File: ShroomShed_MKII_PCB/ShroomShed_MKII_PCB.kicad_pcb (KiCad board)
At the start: 4 copper layers, 70 x 70 mm, 69 parts, among them J1 SWD 14 pin header, J2 TYPE-C-31-M-12, J3 Fan, J4 AUX_SPI, J5 SD_SPI, J6 DHT_I2C, J7 Display_Touch_SPI, J8 Transducer Driver, J9 Control_Panel, Q1 T2N7002AK, Q2 BC817, SW1 EVQ-Q2B03W, SW2 SW_SPDT, U1 AMS1117-3.3, U2 TPS61085DGK, U3 USBLC6-2SC6, U4 ENS210, U5 STM32H562VGTx, Y1 16MHz

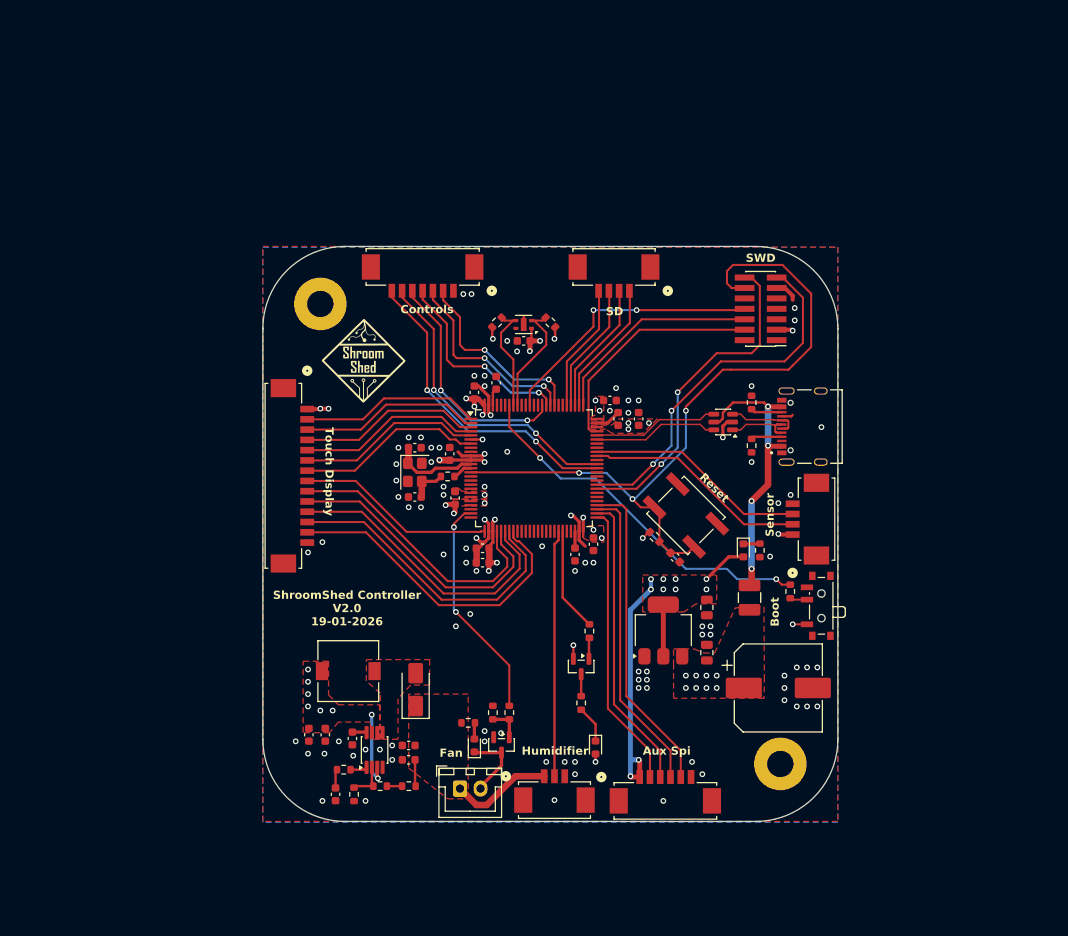
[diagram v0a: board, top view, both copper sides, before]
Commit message: finished V2.1 PCB
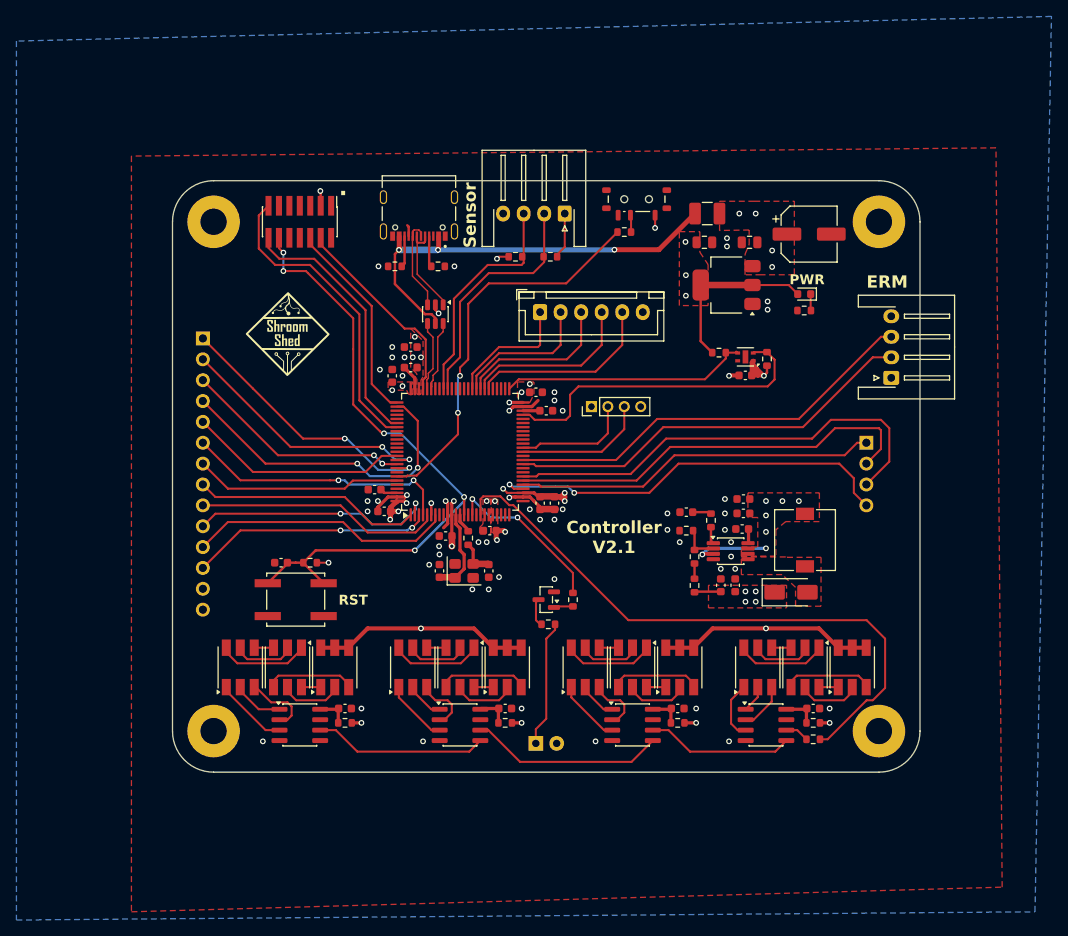
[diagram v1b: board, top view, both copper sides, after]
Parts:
- removed the J4 at (164.0, 132.5)
- removed the J8 at (150.5, 132.4)
- removed J9: Control_Panel, DOWNLOAD_Connectors:CONN_532610001-SD_07_MOL
- removed Q2: BC817, Package_TO_SOT_SMD:SOT-23
- removed the R7 at (150.0, 74.2)
- added C2: 1uF, Capacitor_SMD:C_0603_1608Metric, F.Cu at (182.0, 121.3)
- added C3: 1uF, Capacitor_SMD:C_0603_1608Metric, F.Cu at (125.0, 121.3)
- added C7: 1uF, Capacitor_SMD:C_0603_1608Metric, F.Cu at (165.5, 121.3)
- added C8: 1uF, Capacitor_SMD:C_0603_1608Metric, F.Cu at (144.5, 121.3)
- added D1: XL-5050RGBC, LED_SMD:LED_RGB_5050-6, F.Cu at (186.8, 116.2)
- added D10: XL-5050RGBC, LED_SMD:LED_RGB_5050-6, F.Cu at (154.3, 116.3)
- added D11: XL-5050RGBC, LED_SMD:LED_RGB_5050-6, F.Cu at (144.7, 116.3)
- added D12: XL-5050RGBC, LED_SMD:LED_RGB_5050-6, F.Cu at (139.0, 116.3)
- added D13: XL-5050RGBC, LED_SMD:LED_RGB_5050-6, F.Cu at (133.2, 116.3)
- added D14: BLUE, LED_THT:LED_D4.0mm, B.Cu at (148.2, 125.5)
- added D2: XL-5050RGBC, LED_SMD:LED_RGB_5050-6, F.Cu at (181.0, 116.2)
- added D5: XL-5050RGBC, LED_SMD:LED_RGB_5050-6, F.Cu at (118.0, 116.2)
- added D6: XL-5050RGBC, LED_SMD:LED_RGB_5050-6, F.Cu at (112.2, 116.2)
- added D8: XL-5050RGBC, LED_SMD:LED_RGB_5050-6, F.Cu at (165.8, 116.3)
- added D9: XL-5050RGBC, LED_SMD:LED_RGB_5050-6, F.Cu at (160.0, 116.3)
- added H1: MountingHole_Pad, MountingHole:MountingHole_3.2mm_M3_Pad, F.Cu at (190.0, 62.0)
- added H4: MountingHole_Pad, MountingHole:MountingHole_3.2mm_M3_Pad, F.Cu at (109.0, 124.0)
- added J2: UART, Connector_PinHeader_2.00mm:PinHeader_1x04_P2.00mm_Vertical, F.Cu at (155.0, 84.5)
- added J6: ERM, Connector_JST:JST_XH_S4B-XH-A-1_1x04_P2.50mm_Horizontal, F.Cu at (191.5, 81.0)
- added R1: 33r, Resistor_SMD:R_0603_1608Metric, F.Cu at (182.0, 125.0)
- added R11: 4k7, Resistor_SMD:R_0603_1608Metric, F.Cu at (144.5, 123.0)
- added R20: 10k, Resistor_SMD:R_0603_1608Metric, F.Cu at (145.8, 66.2)
- added R3: 4k7, Resistor_SMD:R_0603_1608Metric, F.Cu at (182.0, 123.0)
- added R4: 4k7, Resistor_SMD:R_0603_1608Metric, F.Cu at (125.0, 123.0)
- added U1: WS2811, Package_SO:SOIC-8_3.9x4.9mm_P1.27mm, F.Cu at (176.2, 123.2)
- added U2: WS2811, Package_SO:SOIC-8_3.9x4.9mm_P1.27mm, F.Cu at (119.5, 123.2)
- added U5: WS2811, Package_SO:SOIC-8_3.9x4.9mm_P1.27mm, F.Cu at (160.0, 123.2)
- added U6: WS2811, Package_SO:SOIC-8_3.9x4.9mm_P1.27mm, F.Cu at (139.0, 123.2)
- C15: renamed from C11; value 1000uF -> 470uF; footprint Capacitor_SMD:CP_Elec_10x10.5 -> Capacitor_SMD:CP_Elec_6.3x7.7
- D3: value Blue -> XL-5050RGBC; footprint LED_SMD:LED_0603_1608Metric -> LED_SMD:LED_RGB_5050-6
- D4: value Yellow -> XL-5050RGBC; footprint LED_SMD:LED_0603_1608Metric -> LED_SMD:LED_RGB_5050-6
- J3: value Fan -> Inputs; footprint Connector_JST:JST_XH_B2B-XH-A_1x02_P2.50mm_Vertical -> Connector_JST:JST_XH_B6B-XH-A_1x06_P2.50mm_Vertical
- J4: renamed from J6; value DHT_I2C -> SHT31; footprint DOWNLOAD_Connectors:CONN_532610001-SD_04_MOL -> Connector_JST:JST_XH_S4B-XH-A-1_1x04_P2.50mm_Horizontal
- J7: renamed from J5; footprint DOWNLOAD_Connectors:CONN_532610001-SD_04_MOL -> Connector_PinSocket_2.54mm:PinSocket_1x04_P2.54mm_Vertical; moved to B.Cu
- J8: renamed from J7; footprint DOWNLOAD_Connectors:CONN_532610001-SD_14_MOL -> Connector_PinSocket_2.54mm:PinSocket_1x14_P2.54mm_Vertical; moved to B.Cu
- Q1: value T2N7002AK -> BC817
- R10: value 2k2 -> 4k7
- R12: value 1k -> 5k1
- R13: value 330r -> 5k1
- R15: value 100R -> 1k
- R16: value 10k -> 500r
- R17: value 2k2 -> 10k
- R18: renamed from R9; value 47r -> 33r
- SW2: value SW_SPDT -> BOOT SELECT; footprint Button_Switch_SMD:SW_SPDT_PCM12 -> Button_Switch_SMD:SW_SPDT_Shouhan_MSK12C02
- moved H2 95.5 mm to (109.0, 62.0)
- moved H3 85.6 mm to (190.0, 124.0)
- moved C1 60.2 mm to (173.5, 95.8), turned to 0 degrees
- moved J3 58.8 mm to (148.8, 73.0)
- moved L1 57.8 mm to (181.0, 100.8), turned to -90 degrees
- moved C4 57.6 mm to (173.5, 97.5), turned to 0 degrees
- moved J5 57.1 mm to (119.5, 62.0), turned to -90 degrees
- moved J1 56.3 mm to (134.0, 59.0), turned to 180 degrees
- moved C15 55.4 mm to (181.5, 63.5)
- moved C6 54.8 mm to (166.6, 97.3), turned to 0 degrees
- moved R12 54.4 mm to (170.5, 77.9), turned to 180 degrees
- moved SW2 54.2 mm to (160.5, 59.2), turned to 180 degrees
- moved R5 54.0 mm to (169.6, 98.3), turned to 90 degrees
- moved C5 53.9 mm to (173.3, 99.4), turned to 0 degrees
- moved R10 53.5 mm to (165.5, 123.0), turned to 180 degrees
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- renumbered C12 to C1, C15 to C10, C10 to C11, C20 to C12, C21 to C13, C22 to C14, C8 to C16, C9 to C17, C23 to C18, C24 to C19, C7 to C20, C1 to C21, C16 to C22, C2 to C23, C3 to C24, C17 to C25, C4 to C26, C5 to C27, C6 to C28, C13 to C4, C18 to C5, C19 to C6, C14 to C9, D1 to D15, D2 to D7, H1 to H3, J2 to J1, J1 to J5, R3 to R14, R14 to R19, R8 to R2, R4 to R21, R11 to R6, R1 to R7, R6 to R8, R2 to R9, U2 to U3, U3 to U4, U4 to U7, U1 to U8, U5 to U9
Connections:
- D3 pad 1: Net-(D3-K) -> Net-(D3-RK)
- D3 pad 2: +5V -> Net-(D3-GK)
- D4 pad 1: Net-(D4-K) -> Net-(D4-RK)
- D4 pad 2: Net-(D4-A) -> Net-(D4-GK)
- J3 pad 1: +12V -> ENCODER_CHANNEL_A
- J3 pad 2: Net-(D4-K) -> ENCODER_CHANNEL_B
- J7 pad 1: SD_NSS -> SD_SCK
- J7 pad 2: SD_SCK -> SD_MISO
- J7 pad 3: SD_MISO -> SD_MOSI
- J7 pad 4: SD_MOSI -> SD_NSS
- J8 pad 1: +3V3 -> TOUCH_IRQ
- J8 pad 10: TOUCH_SCK -> DISPLAY_DC
- J8 pad 11: TOUCH_MISO -> DISPLAY_RST
- J8 pad 12: TOUCH_MOSI -> DISPLAY_NSS
- J8 pad 13: TOUCH_IRQ -> GND
- J8 pad 14: GND -> +3V3
- J8 pad 2: DISPLAY_SCK -> TOUCH_MISO
- J8 pad 3: DISPLAY_DC -> TOUCH_MOSI
- J8 pad 4: DISPLAY_NSS -> TOUCH_NSS
- J8 pad 5: DISPLAY_MISO -> TOUCH_SCK
- J8 pad 6: DISPLAY_MOSI -> DISPLAY_MISO
- J8 pad 7: DISPLAY_RST -> DISPLAY_LED
- J8 pad 8: DISPLAY_LED -> DISPLAY_SCK
- J8 pad 9: TOUCH_NSS -> DISPLAY_MOSI
- Q1 pad 1: Net-(Q1-G) -> Net-(Q1-B)
- Q1 pad 3: Net-(D4-K) -> Net-(Q1-C)
- R10 pad 1: ENS210_SDA -> +12V
- R10 pad 2: +3V3 -> Net-(U5-VDD)
- R12 pad 1: +12V -> ENS210_SDA
- R12 pad 2: Net-(D4-A) -> +3V3
- R13 pad 1: Net-(Q2-C) -> ENS210_SCL
- R13 pad 2: Net-(D3-K) -> +3V3
- R15 pad 1: Net-(Q1-G) -> Net-(Q1-B)
- R15 pad 2: FAN_PWM -> WATER_LED
- R16 pad 1: GND -> Net-(D14-K)
- R16 pad 2: Net-(Q1-G) -> Net-(Q1-C)
- R17 pad 1: Net-(Q2-B) -> +3V3
- R17 pad 2: LED_HUMIDIFIER -> SHT31_SDA
- U9 pad 16: unconnected-(U5-PC1-Pad16) -> WATER_LED
- U9 pad 18: unconnected-(U5-PC3-Pad18) -> RGB_MOSI
- U9 pad 24: FAN_PWM -> unconnected-(U9-PA1-Pad24)
- U9 pad 25: FAN_DETECT -> unconnected-(U9-PA2-Pad25)
- U9 pad 26: DISPLAY_LED -> unconnected-(U9-PA3-Pad26)
- U9 pad 29: TOUCH_NSS -> SD_NSS
- U9 pad 30: TOUCH_SCK -> SD_SCK
- U9 pad 31: TOUCH_MISO -> SD_MISO
- U9 pad 32: TOUCH_MOSI -> SD_MOSI
- U9 pad 33: TOUCH_IRQ -> unconnected-(U9-PC4-Pad33)
- U9 pad 35: unconnected-(U5-PB0-Pad35) -> TRANSDUCER_PWM
- U9 pad 36: unconnected-(U5-PB1-Pad36) -> FAN_PWM
- U9 pad 38: unconnected-(U5-PE7-Pad38) -> RF_RX
- U9 pad 39: unconnected-(U5-PE8-Pad39) -> RF_TX
- U9 pad 44: TRANSDUCER_PWM -> unconnected-(U9-PE13-Pad44)
- U9 pad 45: LED_HUMIDIFIER -> unconnected-(U9-PE14-Pad45)
- U9 pad 47: unconnected-(U5-PB10-Pad47) -> ENS210_SCL
- U9 pad 51: SPI2_NSS -> ENS210_SDA
- U9 pad 52: SPI2_SCK -> unconnected-(U9-PB13-Pad52)
- U9 pad 53: SPI2_MISO -> unconnected-(U9-PB14-Pad53)
- U9 pad 54: SPI2_MOSI -> unconnected-(U9-PB15-Pad54)
- U9 pad 56: unconnected-(U5-PD9-Pad56) -> INPUT_3
- U9 pad 57: unconnected-(U5-PD10-Pad57) -> INPUT_2
- U9 pad 58: UART4_RX -> INPUT_1
- U9 pad 59: UART4_TX -> ENCODER_CHANNEL_B
- U9 pad 60: unconnected-(U5-PD13-Pad60) -> ENCODER_CHANNEL_A
- U9 pad 63: ENCODER_CHANNEL_B -> unconnected-(U9-PC6-Pad63)
- U9 pad 64: ENCODER_CHANNEL_A -> unconnected-(U9-PC7-Pad64)
- U9 pad 77: SD_NSS -> TOUCH_NSS
- U9 pad 78: SD_SCK -> unconnected-(U9-PC10-Pad78)
- U9 pad 79: SD_MISO -> unconnected-(U9-PC11-Pad79)
- U9 pad 80: SD_MOSI -> unconnected-(U9-PC12-Pad80)
- U9 pad 81: unconnected-(U5-PD0-Pad81) -> UART4_RX
- U9 pad 82: unconnected-(U5-PD1-Pad82) -> UART4_TX
- U9 pad 83: LED_WATER -> unconnected-(U9-PD2-Pad83)
- U9 pad 84: BUTTON_2 -> unconnected-(U9-PD3-Pad84)
- U9 pad 85: BUTTON_1 -> unconnected-(U9-PD4-Pad85)
- U9 pad 86: ENCODER_BUTTON -> unconnected-(U9-PD5-Pad86)
- U9 pad 89: SWD_SWO -> TOUCH_SCK
- U9 pad 90: unconnected-(U5-PB4(NJTRST)-Pad90) -> TOUCH_MISO
- U9 pad 91: unconnected-(U5-PB5-Pad91) -> TOUCH_MOSI
- U9 pad 92: ENS210_SCL -> TOUCH_IRQ
- U9 pad 93: ENS210_SDA -> unconnected-(U9-PB7-Pad93)
- U9 pad 95: unconnected-(U5-PB8-Pad95) -> DISPLAY_LED
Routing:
- net RGB_MOSI: track 0.00 -> 75.0 mm
- net +12V: track 15.8 -> 61.5 mm, vias 0 -> 10
- net SD_MOSI: track 15.4 -> 55.9 mm
- net SPI2_MOSI: track 39.1 -> 0.00 mm
- net SPI2_MISO: track 37.7 -> 0.00 mm
- net SPI2_SCK: track 36.2 -> 0.00 mm
- net SD_MISO: track 15.8 -> 51.1 mm
- net SPI2_NSS: track 34.8 -> 0.00 mm
- net SD_NSS: track 16.4 -> 50.3 mm, vias 0 -> 2
- net SWD_SWO: track 33.2 -> 0.00 mm, vias 2 -> 0
- net ENCODER_BUTTON: track 28.7 -> 0.00 mm, vias 2 -> 0
- net SD_SCK: track 16.1 -> 44.1 mm
- net ENS210_SCL: track 14.6 -> 39.8 mm
- net BUTTON_1: track 24.5 -> 0.00 mm, vias 2 -> 0
- net BUTTON_2: track 24.1 -> 0.00 mm, vias 2 -> 0
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- added copper zone on In2.Cu, net +12V
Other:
- board size 70 x 70 mm -> 91 x 72 mm
- board text added: "."
- board text added: "Controller V2.1"
- board text added: "ERM"
- board text added: "PWR"
- board text added: "RST"
- board text removed: "Aux Spi"
- board text removed: "Boot"
- board text removed: "Controls"
- board text removed: "Fan"
- board text removed: "Humidifier"
- board text removed: "Reset"
- board text removed: "SD"
- board text removed: "SWD"
- board text removed: "ShroomShed Controller V2.0 19-01-2026"
- board text removed: "Touch Display"
